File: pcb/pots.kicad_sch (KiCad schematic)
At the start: 9 parts, among them SW1 DSHP03TSGET

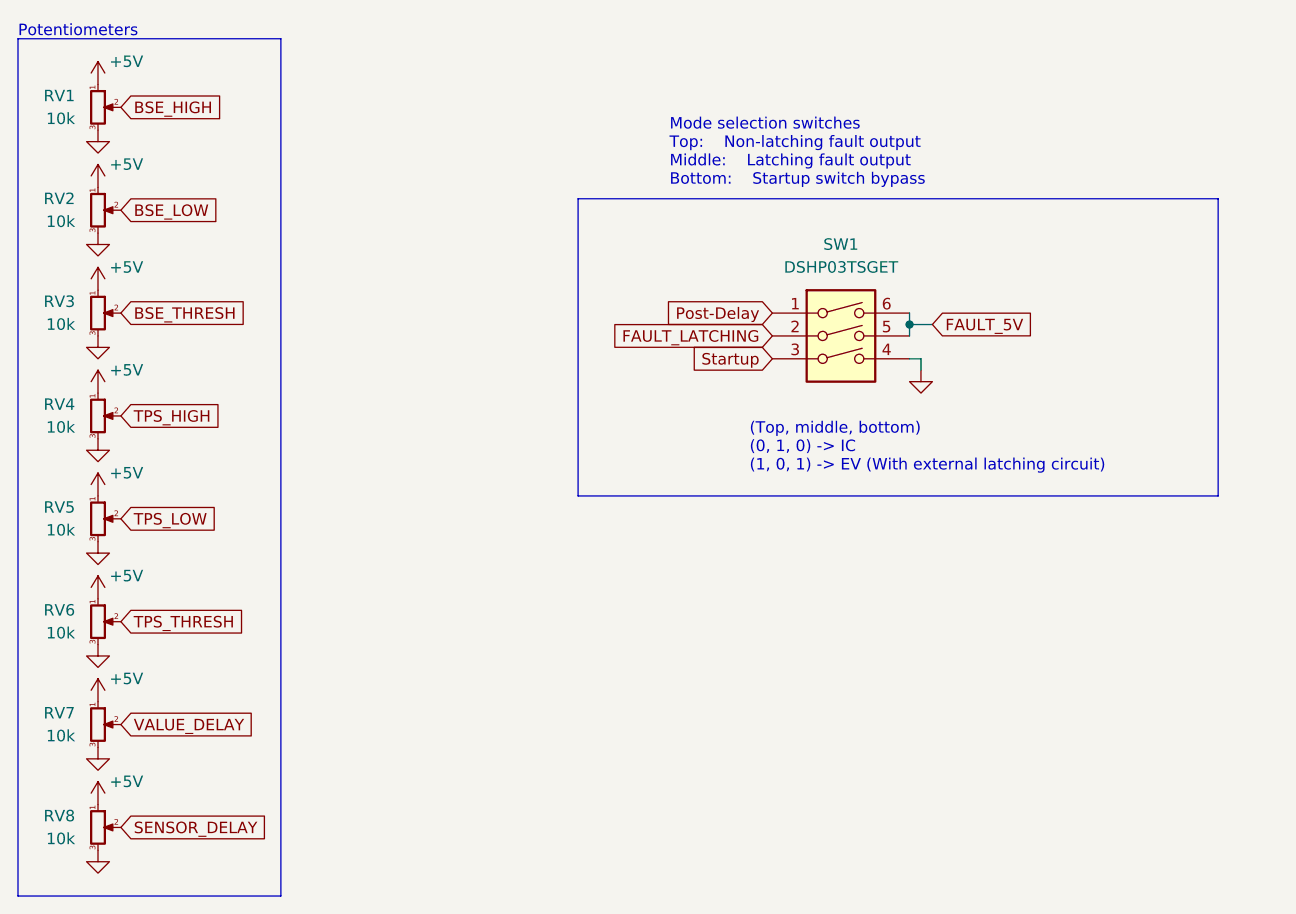
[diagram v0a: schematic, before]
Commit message: CI/CD Changes
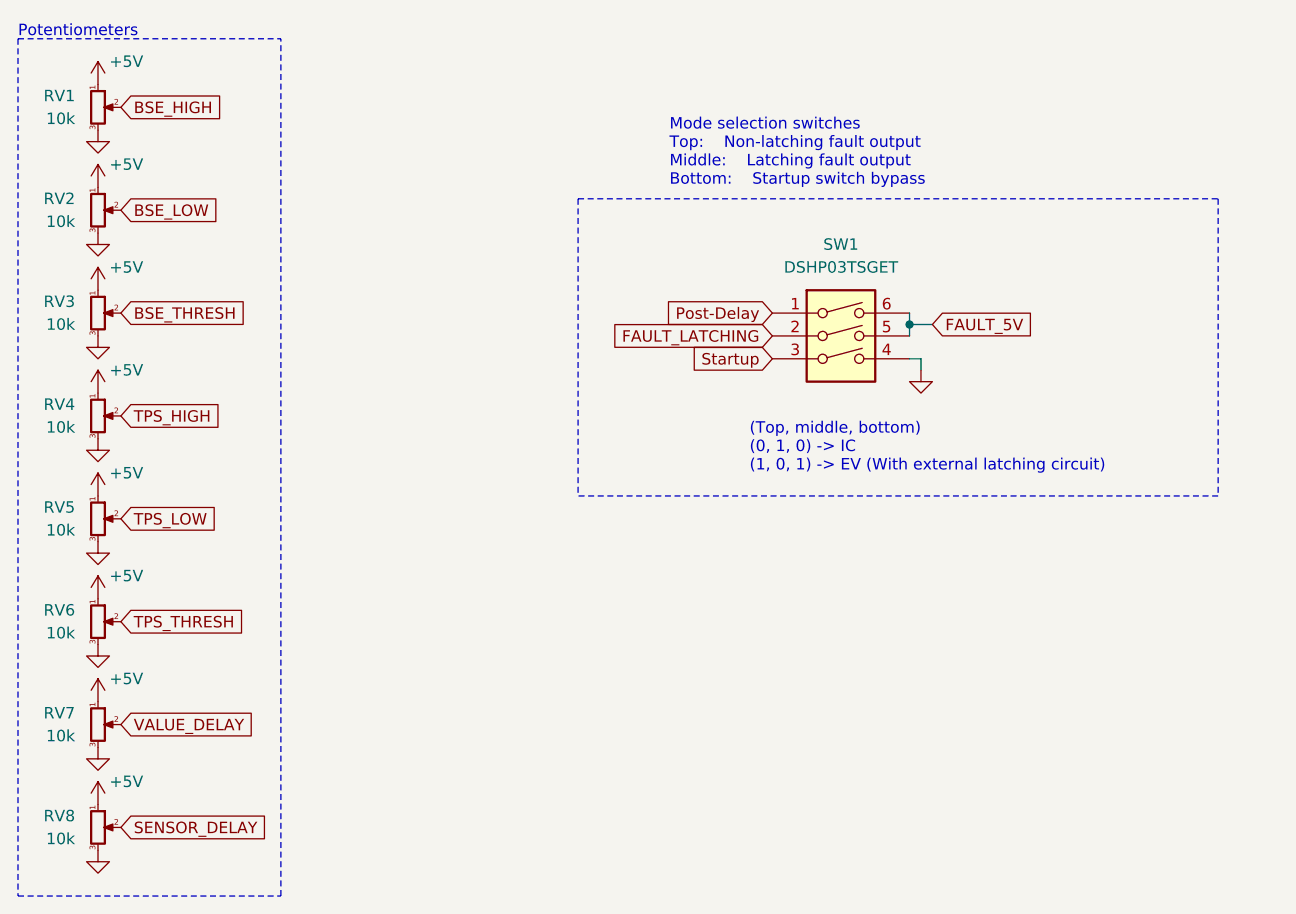
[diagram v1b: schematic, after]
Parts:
- RV1, RV2, RV3, RV4, RV5, RV6, RV7, RV8: Spice_Lib_File SPICE models/pot.lib -> (none); Spice_Model Potentiometer -> (none); Spice_Netlist_Enabled Y -> (none); Spice_Primitive X -> (none)
